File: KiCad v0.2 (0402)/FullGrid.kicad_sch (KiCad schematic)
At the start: 202 parts, among them J1 Conn_01x16

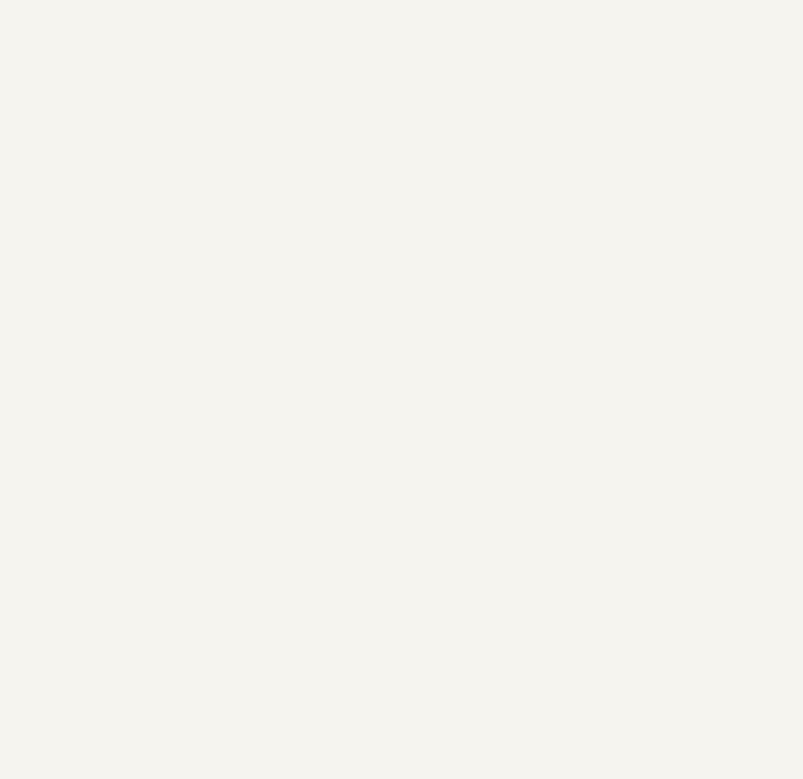
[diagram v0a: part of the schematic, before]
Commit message: Uhm
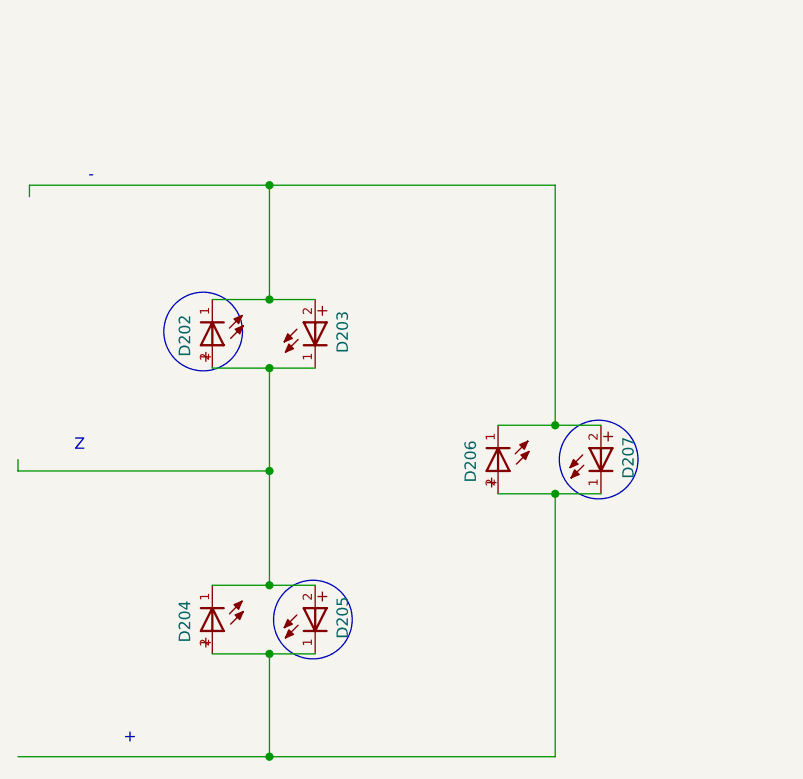
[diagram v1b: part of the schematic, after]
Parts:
- added D202, D203, D204, D205, D206, D207: WL-SMCC_0402, WL-SMCC_0402:WL-SMCC_0402, symbol WL-SMCC_0402:WL-SMCC_0402
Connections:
- new net: D202.1, D203.2, D206.1, D207.2
- new net: D204.2, D205.1, D206.2, D207.1
- new net: D202.2, D203.1, D204.1, D205.2
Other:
- note added: "+"
- note added: "-"
- note added: "Z"
